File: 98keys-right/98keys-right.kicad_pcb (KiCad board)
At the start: 2 copper layers, 225 x 231 mm, 115 parts, among them J1 Conn_01x04_Male/I2C, SW1 MX-NO-LED, SW10 MX-NO-LED, SW11 MX-NO-LED, SW12 MX-NO-LED, SW13 MX-NO-LED, SW14 MX-NO-LED, SW15 MX-NO-LED, SW16 MX-NO-LED, SW17 MX-NO-LED, SW18 MX-NO-LED, SW19 MX-NO-LED, SW2 MX-NO-LED, SW20 MX-NO-LED, SW21 MX-NO-LED, SW22 MX-NO-LED, SW23 MX-NO-LED, SW24 MX-NO-LED, SW25 MX-NO-LED, SW26 MX-NO-LED, SW27 MX-NO-LED, SW28 MX-NO-LED, SW29 MX-NO-LED, SW3 MX-NO-LED, SW30 MX-NO-LED, SW31 MX-NO-LED, SW32 MX-NO-LED, SW33 MX-NO-LED, SW34 MX-NO-LED, SW35 MX-NO-LED, SW36 MX-NO-LED, SW37 MX-NO-LED, SW38 MX-NO-LED, SW39 MX-NO-LED, SW4 MX-NO-LED, SW40 MX-NO-LED, SW41 MX-NO-LED, SW42 MX-NO-LED, SW43 MX-NO-LED, SW44 MX-NO-LED, SW45 MX-NO-LED, SW46 MX-NO-LED, SW47 MX-NO-LED, SW48 SW_Push/KS-01Q-01, SW5 MX-NO-LED, SW6 MX-NO-LED, SW7 MX-NO-LED, SW8 MX-NO-LED, SW9 MX-NO-LED, U1 Pico

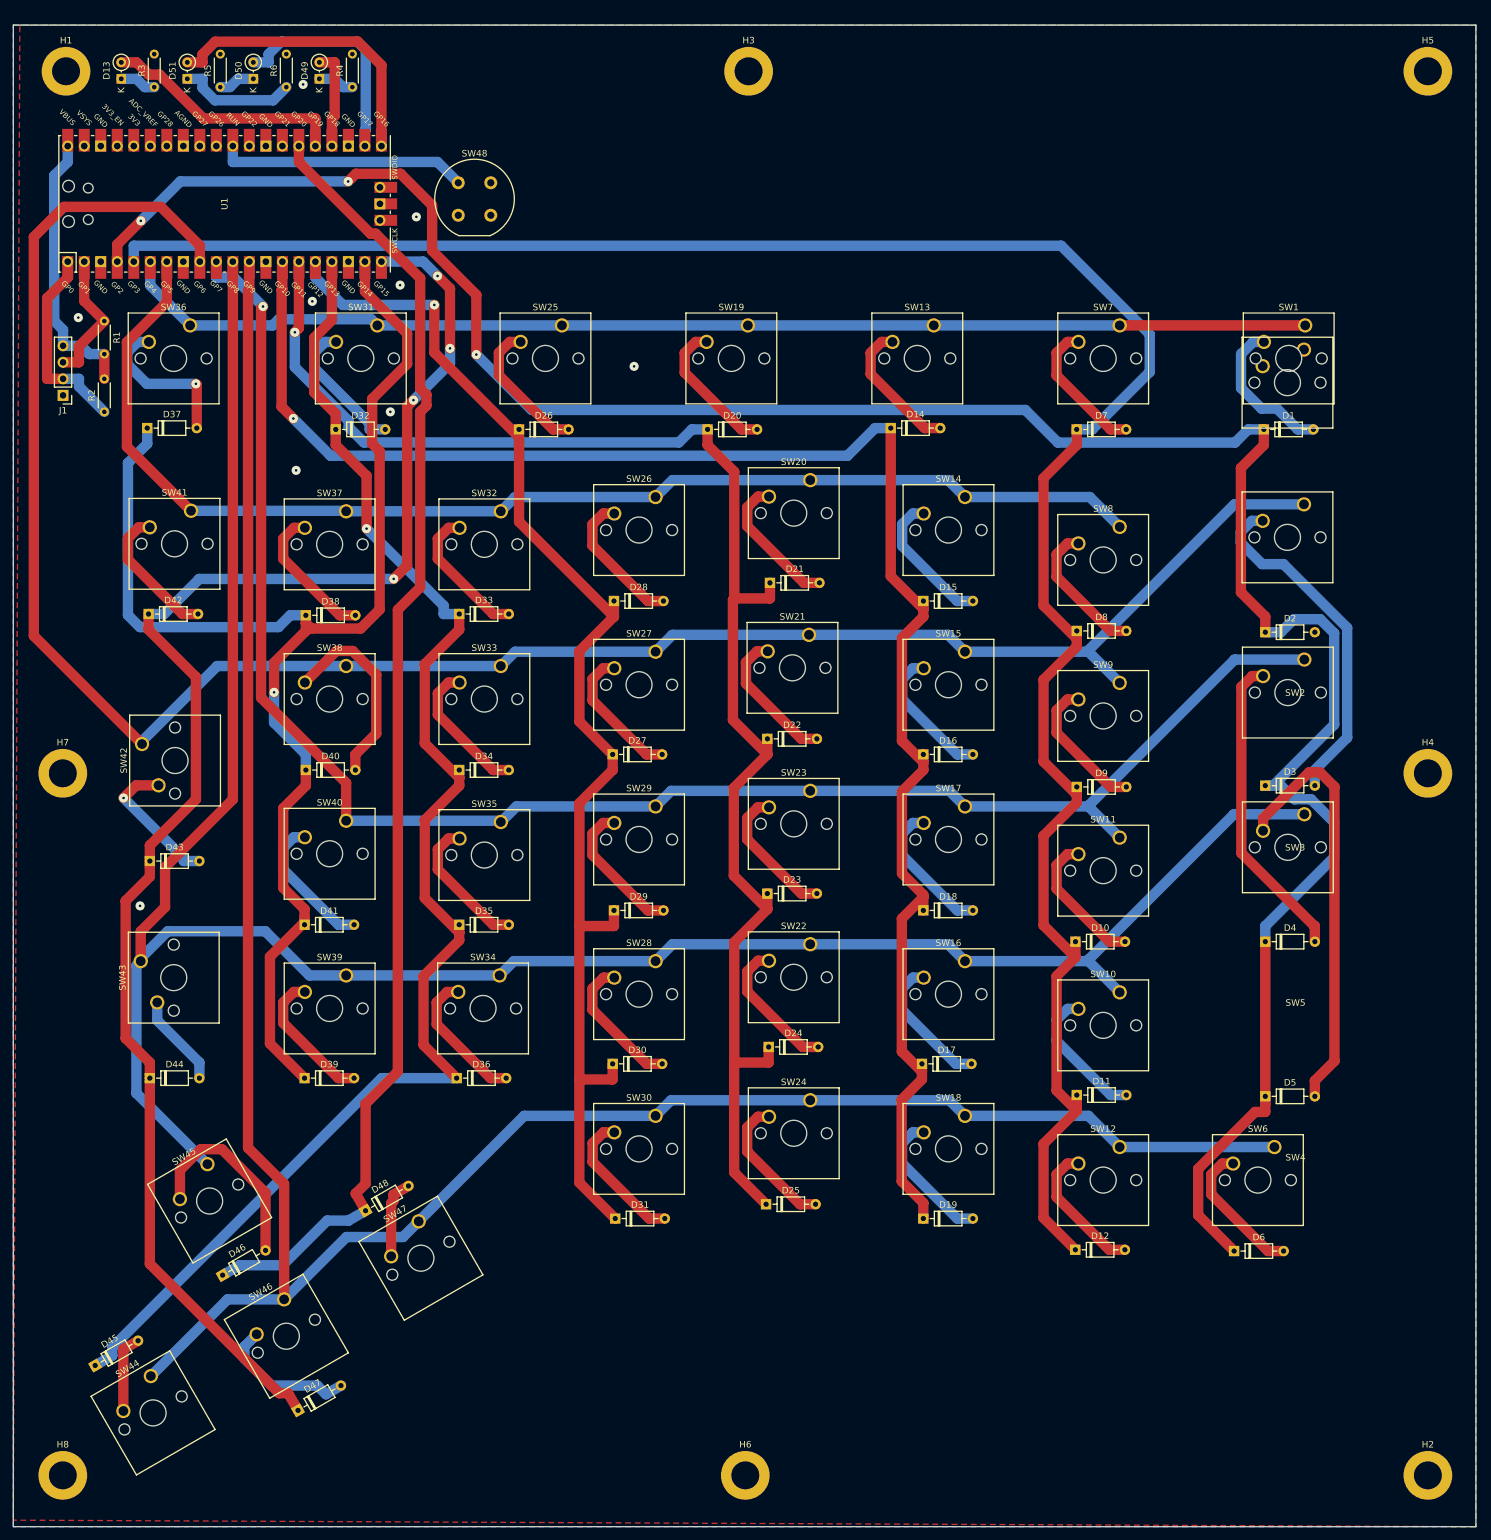
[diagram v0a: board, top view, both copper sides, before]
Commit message: Add files via upload
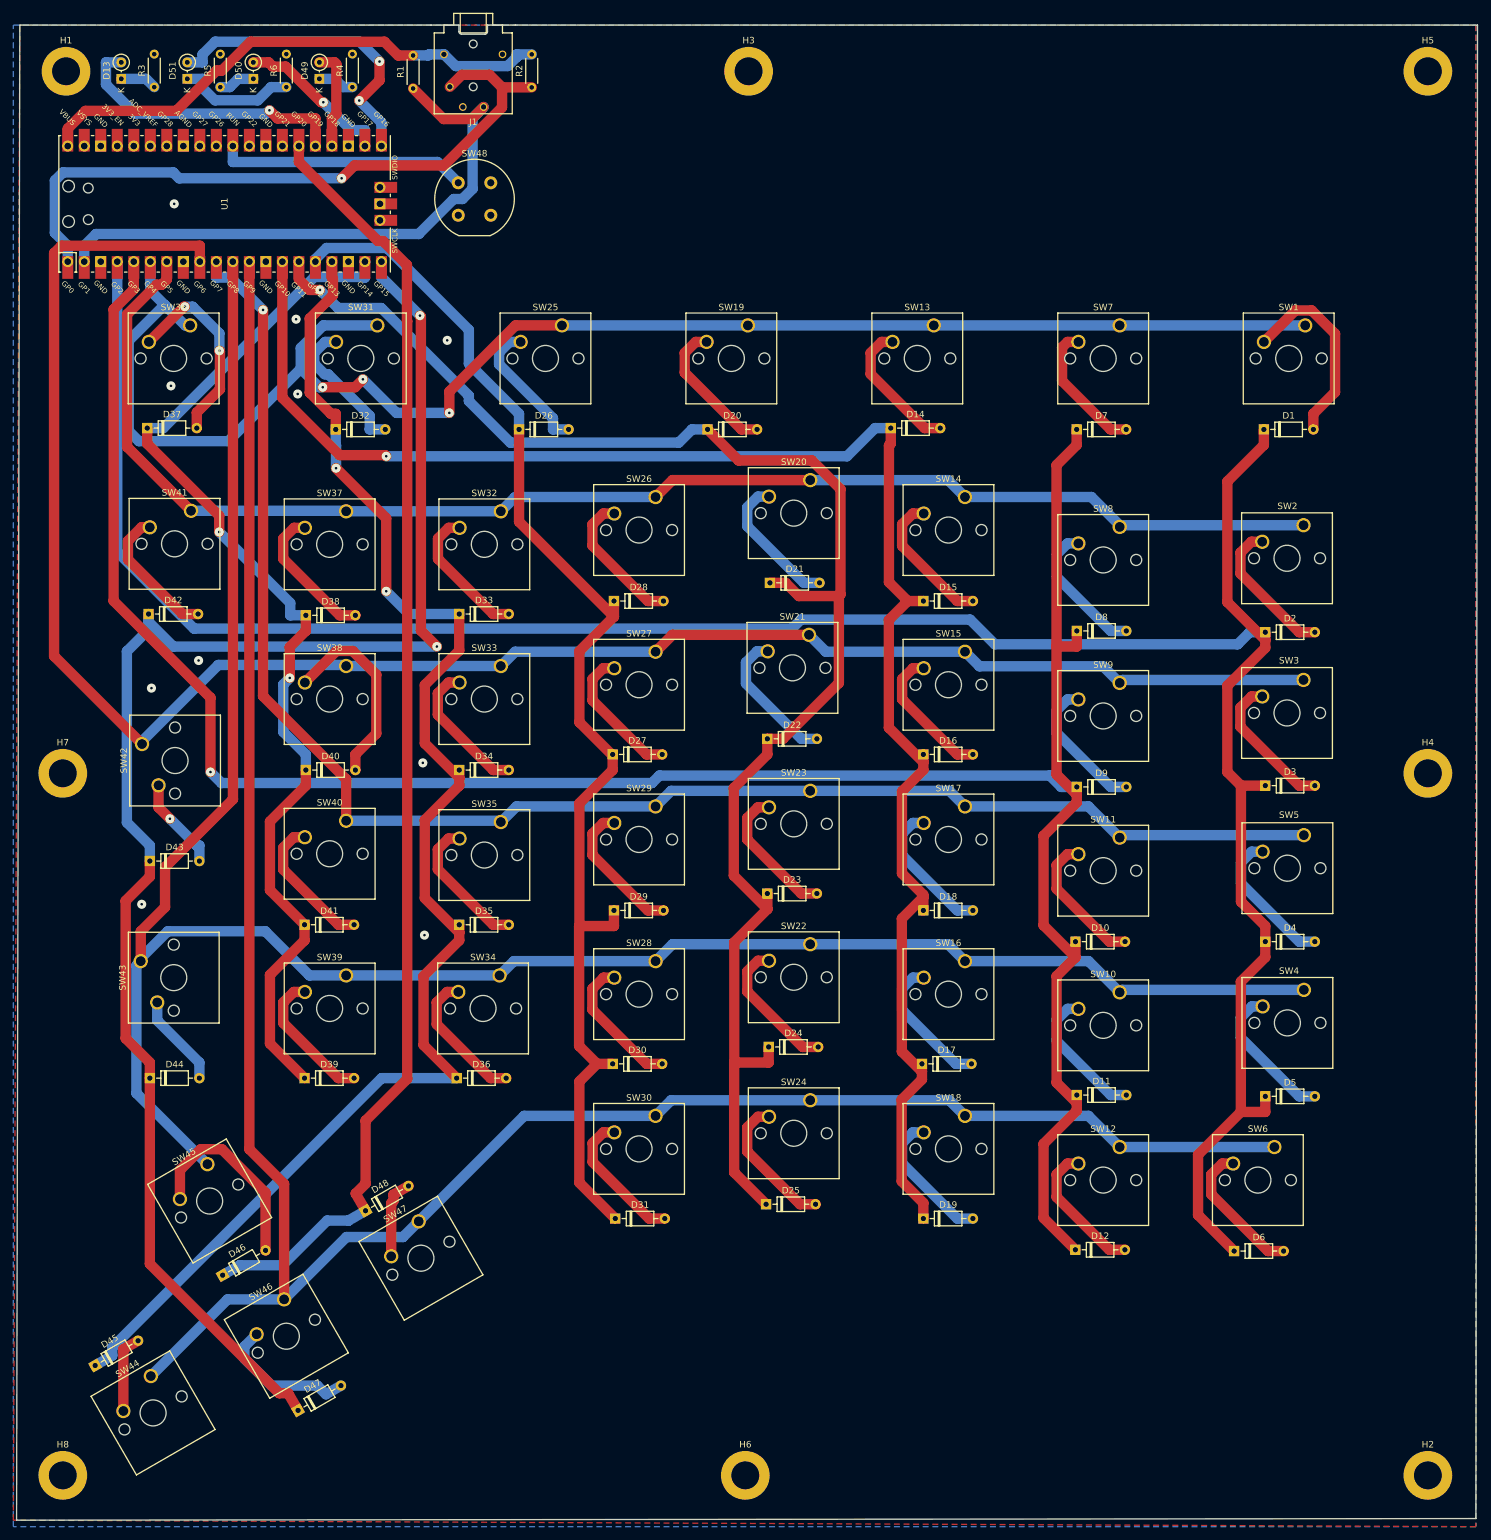
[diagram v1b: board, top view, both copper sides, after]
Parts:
- J1: footprint Connector_PinHeader_2.54mm:PinHeader_1x04_P2.54mm_Vertical -> Connector_Audio:Jack_3.5mm_CUI_SJ1-43514_Horizontal
- moved R2 82.6 mm to (145.8, 32.6)
- moved J1 82.1 mm to (136.8, 27.5)
- moved R1 59.5 mm to (127.5, 32.8), turned to 90 degrees
- moved SW2 27.0 mm to (264.5, 99.9)
- moved SW3 27.0 mm to (264.5, 123.7)
- moved SW5 27.0 mm to (264.5, 147.6)
- moved SW4 27.0 mm to (264.5, 171.4)
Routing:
- net sda: track 30.9 -> 104.8 mm, vias 0 -> 1
- net scl: track 20.8 -> 92.7 mm
- net ROW1: track 184.7 -> 248.5 mm, vias 0 -> 3
- net COL7: track 213.6 -> 168.9 mm, vias 1 -> 2
- net Net-(D5-Pad2): track 65.6 -> 22.3 mm
- net VCC: track 42.8 -> 82.3 mm
- net COL2: track 337.7 -> 371.0 mm, vias 0 -> 1
- net Net-(D3-Pad2): track 53.9 -> 22.2 mm
- net ROW2: track 192.8 -> 221.7 mm
- net Net-(D4-Pad2): track 47.9 -> 22.3 mm
- net ROW3: track 320.6 -> 295.7 mm
- net Net-(D2-Pad2): track 0.00 -> 22.4 mm
- net ROW4: track 262.8 -> 248.1 mm
- net ROW5: track 352.8 -> 338.6 mm
- net PWM2: track 34.7 -> 23.9 mm, vias 0 -> 1
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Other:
- board size 225 x 231 mm -> 224.8 x 230 mm
